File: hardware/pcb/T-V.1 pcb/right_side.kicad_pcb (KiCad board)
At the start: 2 copper layers, 55.8 x 79.5 mm, 16 parts, among them J1 TX HINGE, J2 RX HINGE, J3 GND HINGE, J4 3V3 HINGE, J5 TFT screen, J7 SD READER

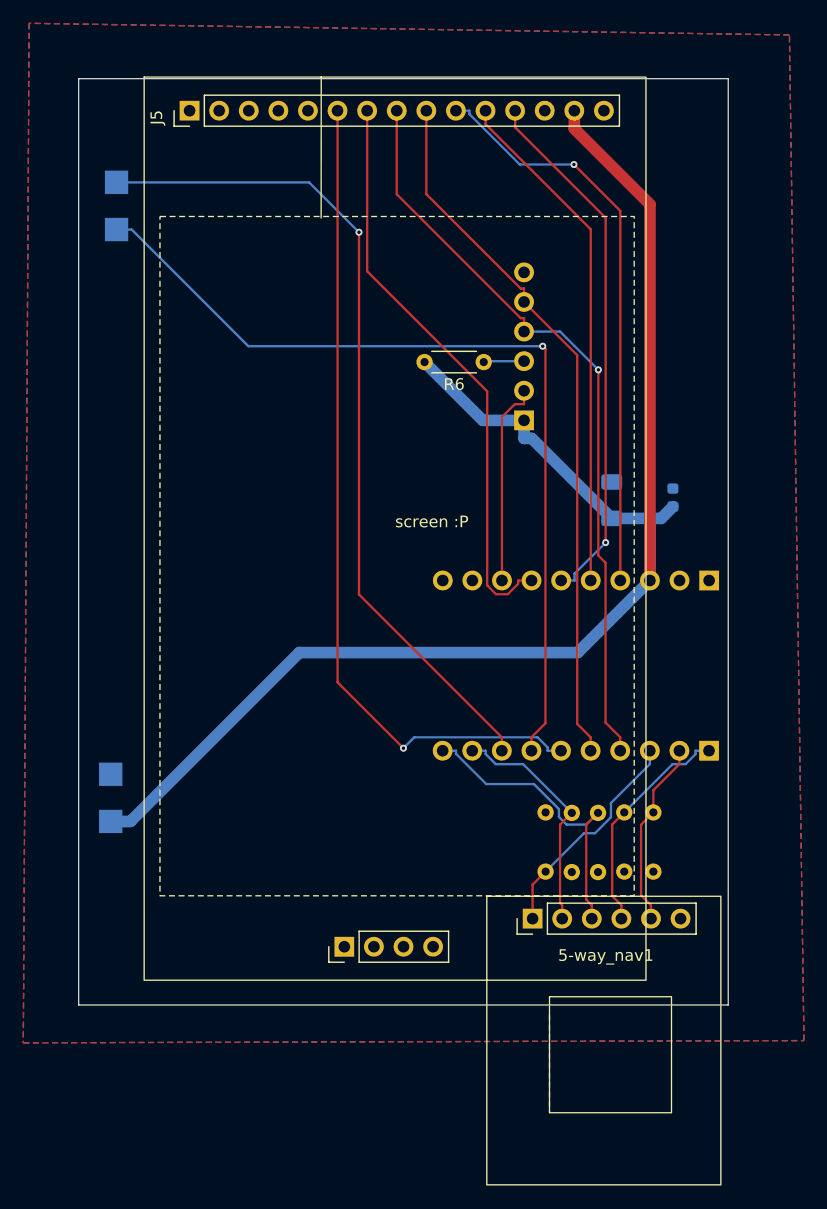
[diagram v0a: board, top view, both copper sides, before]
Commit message: Updating PCB files :P
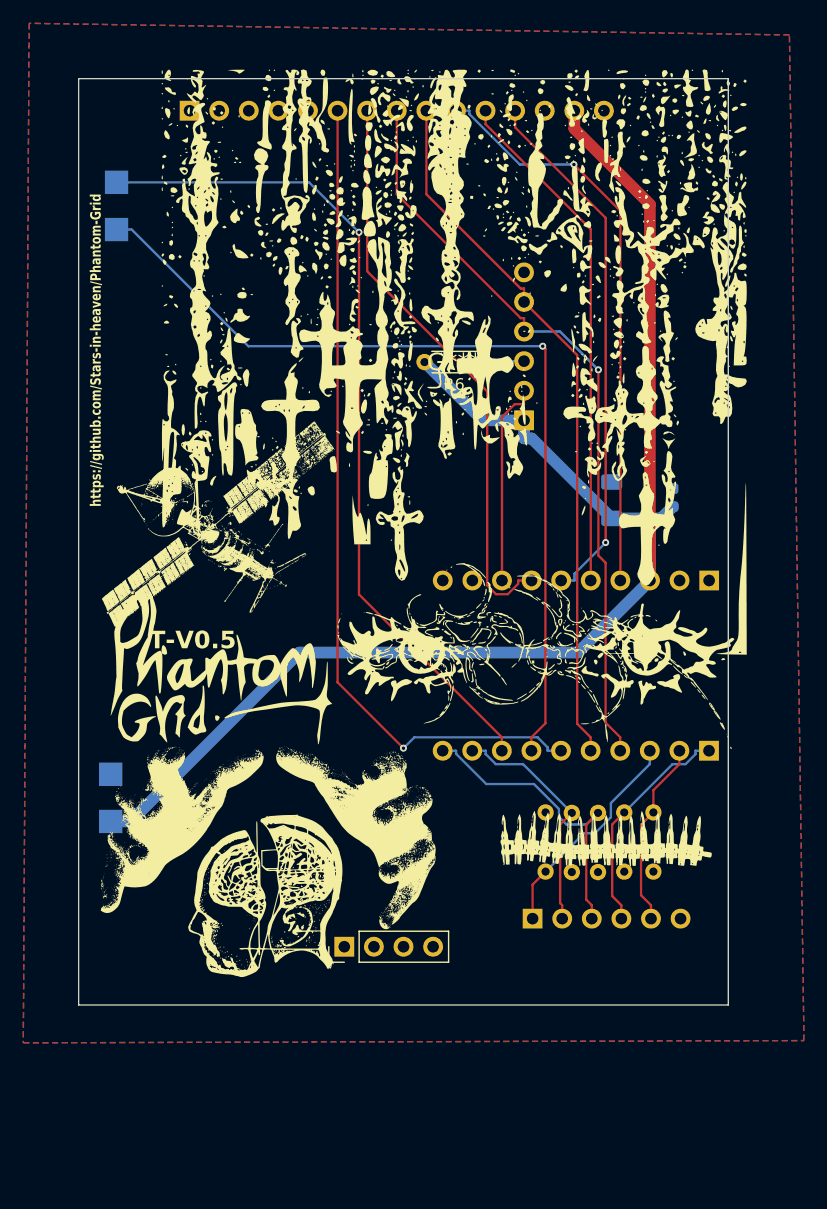
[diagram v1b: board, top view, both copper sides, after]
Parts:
- added .: LOGO, LOGO, F.Cu at (129.5, 82.2)
- added G***: LOGO, LOGO, F.Cu at (106.8, 97.8)
- added G***: LOGO, LOGO, B.Cu at (136.5, 107.0)
- added G***: LOGO, LOGO, B.Cu at (113.2, 101.9)
- added G***: LOGO, LOGO, B.Cu at (96.9, 103.7)
- added G***: LOGO, LOGO, B.Cu at (109.6, 62.2)
- added G***: LOGO, LOGO, F.Cu at (136.0, 98.0)
- added G***: LOGO, LOGO, F.Cu at (106.5, 103.0)
- added G***: LOGO, LOGO, F.Cu at (122.7, 57.1)
- added G***: LOGO, LOGO, F.Cu at (102.5, 71.0)
- added G***: LOGO, LOGO, B.Cu at (114.2, 62.9)
- added G***: LOGO, LOGO, B.Cu at (115.8, 64.4)
- added G***: LOGO, LOGO, B.Cu at (131.9, 98.4)
- added G***: LOGO, LOGO, B.Cu at (128.9, 95.2)
- added logo 2: LOGO, LOGO, F.Cu at (102.4, 83.0)
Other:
- board text added: "T-V0.5"
- board text added: "https://github.com/Stars-in-heaven/Phantom-Grid"
